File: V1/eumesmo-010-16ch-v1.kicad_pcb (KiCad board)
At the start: 4 copper layers, 128 x 67.8 mm, 284 parts, among them J1 250-208, J2 250-208, J3 250-208, J4 250-208, J5 250-202, J6 USB_C_Receptacle_USB2.0, J7 ETHERNET, Q1 WPM2015-3/TR, Q2 MMUN2211LT3G, Q3 UMH3N, SW1 RESET, U1 TX4138, U10 ISO1540, U11 PCA9685PW, U12 MCP23017, U13 TLV274, U14 TLV274, U15 TLV274, U16 TLV274, U2 L78L05_SOT89, U3 B2412S-1WR3, U4 SY8089A1AAC, U5 TPS3820-33, U6 CH340K, U7 ESP32-WROOM-32UE-N16, U8 LAN8710A, U9 TPS3823-33

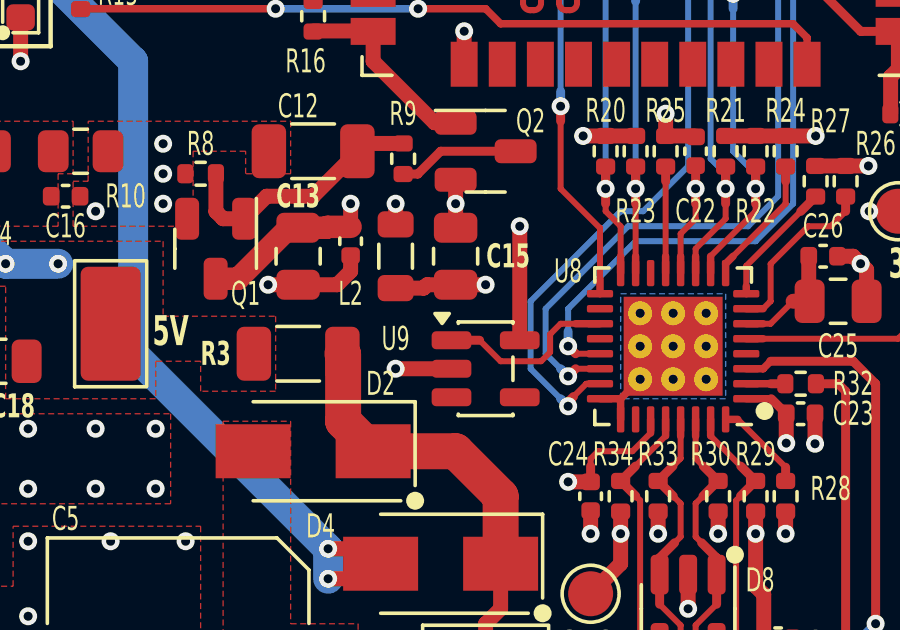
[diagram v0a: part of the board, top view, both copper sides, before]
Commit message: Text translated to english
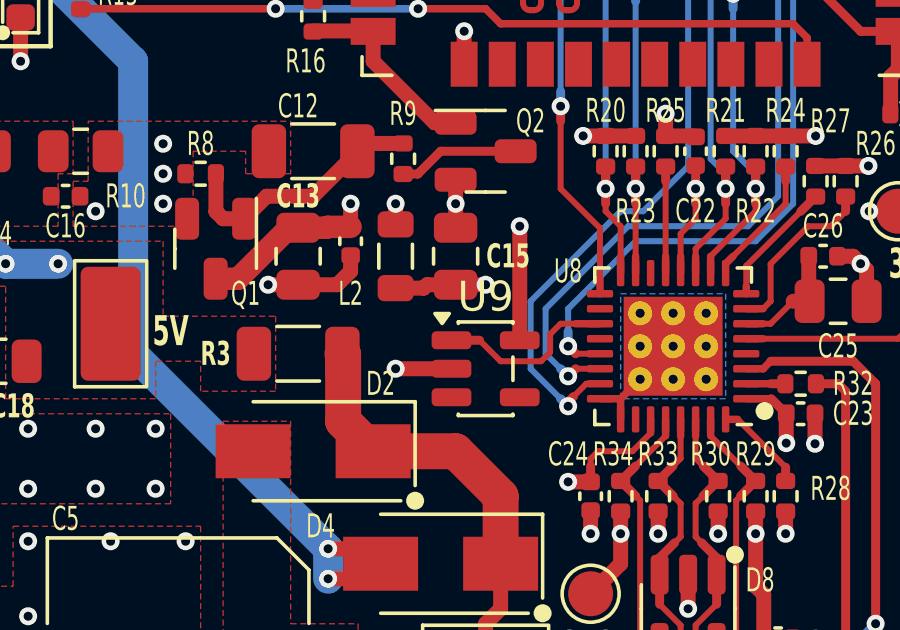
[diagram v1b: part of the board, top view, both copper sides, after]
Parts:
- U9: value TPS3823-33 -> TPS3820-33
